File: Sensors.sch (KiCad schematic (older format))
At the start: 71 parts, among them CN3 CONN_HEADER_SMD_4POS_2MM, CN4 CONN_HEADER_SMD_4POS_2MM, J2 Conn_01x02, U1 LPS25HB, U10 MPXV4006GP, U11 MPXV4006DP, U12 TLV2333IDR, U17 MPXV4006GP, U7 74ACT244PW

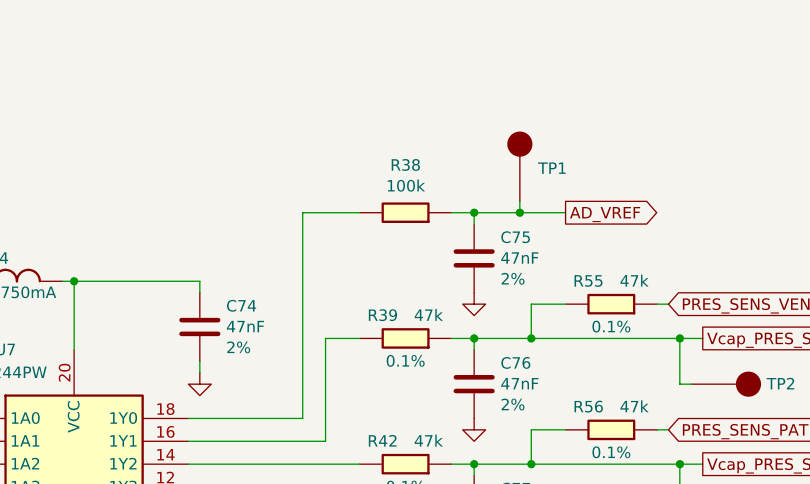
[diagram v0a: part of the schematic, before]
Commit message: Update Sensors.sch
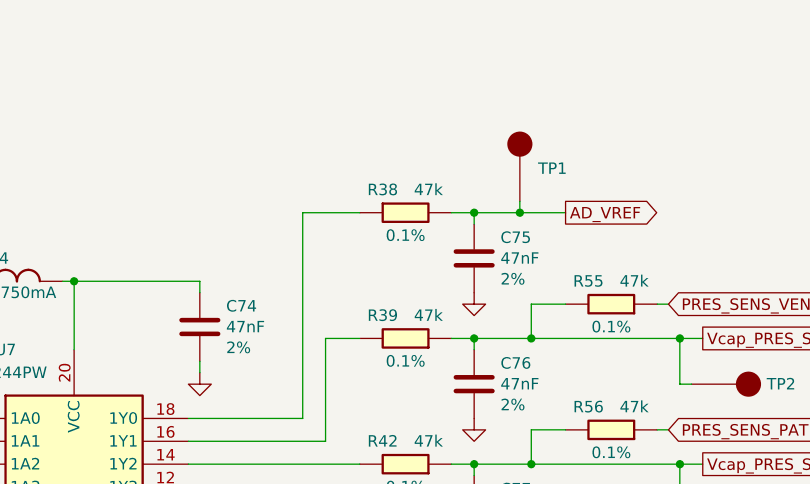
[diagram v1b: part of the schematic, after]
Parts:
- removed R38: 100K_0603_Chip_Resistor,_1%,_0.1W, symbol OpenVent:100K_0603_Chip_Resistor,_1%,_0.1W
- added R38: R_0603_47K_0.1%_0.1W_Film, Resistor_SMD:R_0603_1608Metric_Pad0.98x0.95mm_HandSolder, symbol OpenVent:R_0603_47K_0.1%_0.1W_Film
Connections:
- net AD_VREF: now also R38.2
- net at U7.18 (1Y0): now also R38.1
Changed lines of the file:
@@
 	5800 7100 5800 7150
-$Comp
-L OpenVent:100K_0603_Chip_Resistor,_1%,_0.1W R?
-U 1 1 61F2C4A7
-P 8800 1500
-AR Path="/601B7AF8/61F2C4A7" Ref="R?"  Part="1"
-AR Path="/5F8F3873/61F2C4A7" Ref="R38"  Part="1"
-F 0 "R38" H 8900 1193 50  0000 C CNN
-F 1 "100K_0603_Chip_Resistor,_1%,_0.1W" H 8800 1500 50  0001 C CNN
-F 2 "" H 8800 1500 50  0001 C CNN
-F 3 "" H 8800 1500 50  0001 C CNN
-F 4 "100k" H 8900 1284 50  0000 C CNN "Val"
-F 5 "1%" H 8800 1500 50  0001 C CNN "Tolerance"
-F 6 "0.1W" H 8800 1500 50  0001 C CNN "Watt"
-	1    8800 1500
-	-1   0    0    1
-$EndComp
 $Comp
 L OpenVent:GND #PWR?
@@
 $EndComp
 NoConn ~ 2625 7000
+$Comp
+L OpenVent:R_0603_47K_0.1%_0.1W_Film R38
+U 1 1 60EB5CDA
+P 8600 1300
+F 0 "R38" H 8600 1300 50  0000 C CNN
+F 1 "R_0603_47K_0.1%_0.1W_Film" H 8600 1300 50  0001 C CNN
+F 2 "Resistor_SMD:R_0603_1608Metric_Pad0.98x0.95mm_HandSolder" H 8600 1300 50  0001 C CNN
+F 3 "https://www.digikey.com/en/products/filter/chip-resistor-surface-mount/52" H 8600 1300 50  0001 C CNN
+F 4 "47k" H 8800 1300 50  0000 C CNN "Val"
+F 5 "0.1%" H 8700 1100 50  0000 C CNN "Tolerance"
+F 6 "0.1W" H 8600 1300 50  0001 C CNN "Watt"
+F 7 "KOA Speer Electronics, Inc." H 8600 1300 50  0001 C CNN "Mfr"
+F 8 "RN73H1JTTD4702B25" H 8600 1300 50  0001 C CNN "Mfr_PN"
+F 9 "RES 47K OHM 0.1% 1/10W 0603" H 8600 1300 50  0001 C CNN "Desc"
+F 10 "47 kOhms ±0.1% 0.1W, 1/10W Chip Resistor 0603 (1608 Metric) Automotive AEC-Q200, Moisture Resistant Metal Film" H 8600 1300 50  0001 C CNN "Detailed"
+	1    8600 1300
+	1    0    0    -1
+$EndComp
 $EndSCHEMATC
